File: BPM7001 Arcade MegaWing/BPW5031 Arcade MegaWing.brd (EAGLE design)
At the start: 85.1 x 71.4 mm, 61 parts, among them SW1 TPA-5POS

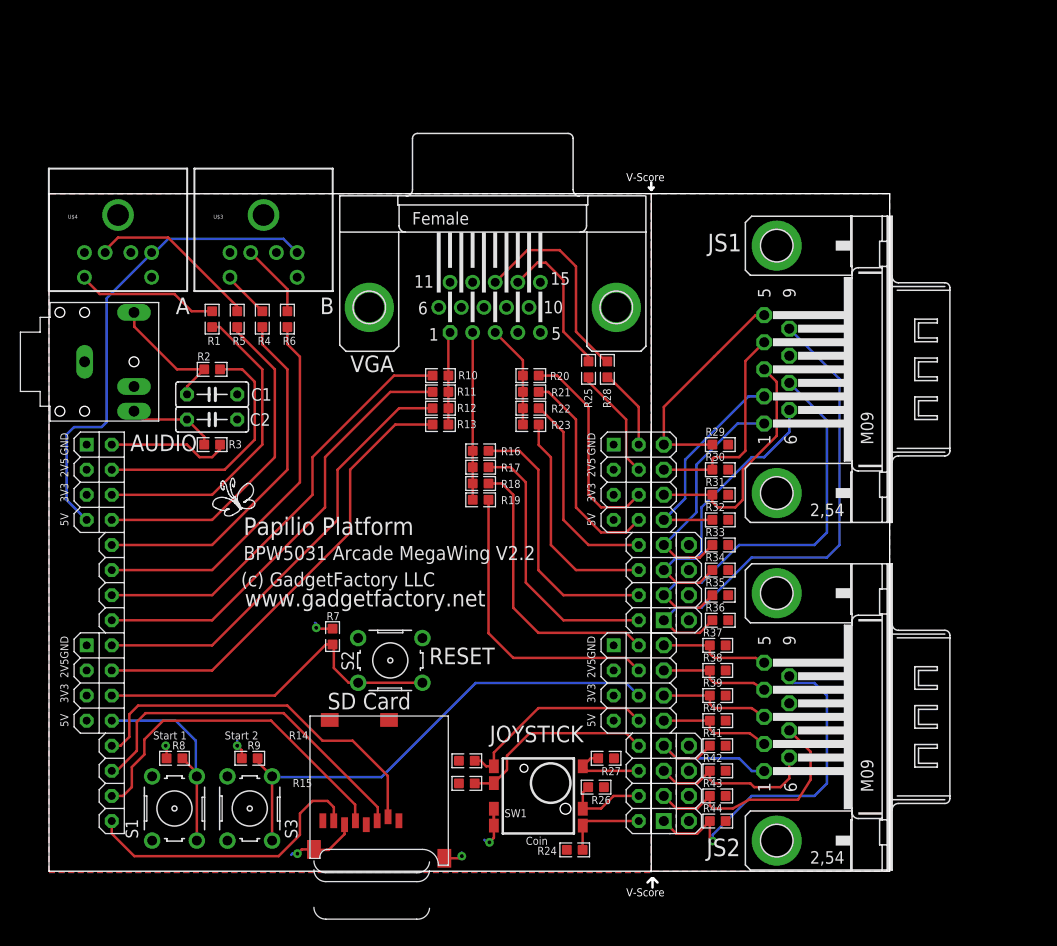
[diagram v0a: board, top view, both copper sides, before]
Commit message: Arcade MegaWing V1.3
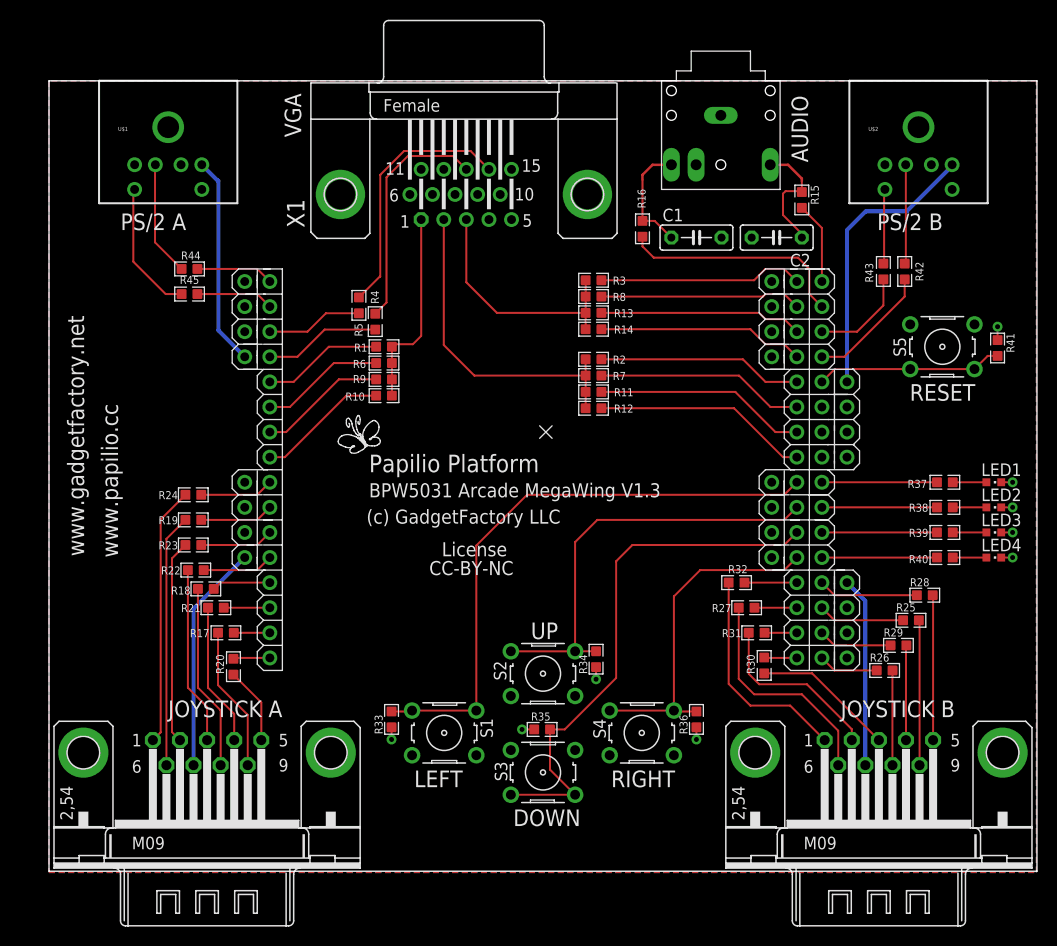
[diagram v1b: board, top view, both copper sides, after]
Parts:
- removed AH, AL: WING8WING8_NOHOLES, Papilio:WINGSIDE_8BIT_NOHOLES
- removed AUDIO1: AUDIOJACK, GadgetFactory:AUDJCK
- removed LOGO1: BUTTERFLY_LOGO, GadgetFactory_Pub:BUTTERFLY_LOGO
- removed SW1: TPA-5POS, GadgetFactory:TPA-5POS
- removed U$3, U$4: MINI-DIN6PTH, SparkFun-Connectors:MINI-DIN6
- added AUDIO: AUDIOJACK, GadgetFactory_6.0:AUDJCK
- added J1: COCOON_48BIT_WINGSIDE, usb1:COCOON_48BIT_WINGSIDE
- added LED1, LED2, LED3, LED4: (no value), led:CHIPLED_0603
- added LOGO2: BUTTERFLY_LOGO, GadgetFactory_Pub:BUTTERFLY_LOGO
- added R45: 390, GadgetFactory:0603
- added S4, S5: (no value), opto:B3F-10XX
- R1: value 390 -> 3.9K
- R10: value 3.9K -> 510
- R11: value 2K -> 1K
- R12: value 1K -> 510
- R13: value 510 -> 1K
- R14: value 47K -> 510
- R15: value 47K -> 3.3K
- R16: value 3.9K -> 3.3K
- R17, R21: value 2K -> 390
- R18, R22: value 1K -> 390
- R19, R23: value 510 -> 390
- R2, R3: value 3.3K -> 3.9K
- R20: value 3.9K -> 390
- R24, R26, R27, R29, R30, R31, R32, R37, R38, R39, R40, R42, R43, R44: value 47K -> 390
- R25, R28: value 82.5 -> 390
- R4, R5: value 390 -> 82.5
- R6: value 390 -> 2K
- R7, R8: value 47K -> 2K
- R9: value 47K -> 1K
- U$1: value MEGAWING_HALF_P1 -> MINI-DIN6PTH; device Papilio:MEGAWING_HALF_NOHOLES_P1 -> SparkFun-Connectors:MINI-DIN6
- U$2: value MICROSD -> MINI-DIN6PTH; device adafruit:MICROSD -> SparkFun-Connectors:MINI-DIN6
- X1: device GadgetFactory:HDF15H -> GadgetFactory_6.0:HDF15H
- moved U$2 89.0 mm to (88.0, 80.0)
- moved U$1 80.9 mm to (12.1, 80.0)
- moved R44 77.3 mm to (14.2, 61.0), turned to 180 degrees
- moved JS1 69.5 mm to (16.0, 12.0), turned to 0 degrees
- moved R15 68.1 mm to (76.2, 67.9), turned to 270 degrees
- moved R8 63.1 mm to (55.1, 58.2), turned to 180 degrees
- moved C2 60.0 mm to (73.7, 64.1), turned to 180 degrees
- moved R43 55.7 mm to (84.5, 60.7), turned to 90 degrees
- moved R42 54.0 mm to (86.6, 60.7), turned to 90 degrees
- moved R24 52.7 mm to (14.6, 38.1), turned to 180 degrees
- moved C1 51.5 mm to (65.5, 64.1)
- moved R41 49.2 mm to (96.0, 53.0), turned to 270 degrees
- moved R14 45.5 mm to (55.1, 54.9), turned to 180 degrees
- moved R20 42.1 mm to (18.7, 20.7), turned to 270 degrees
- moved R3 42.0 mm to (55.1, 59.8), turned to 180 degrees
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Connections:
- removed net BLUE0: R20.1, U$1.A19
- removed net GREEN0: R16.1, U$1.A23
- removed net JOY_3V3: AH.3V3@2, AL.3V3@2, R29.2, R30.2, R31.2, R32.2, R33.2, R34.2, R35.2, R36.2, R37.2, R38.2, R39.2, R40.2, R41.2, R42.2, R43.2, R44.2
- removed net JOY_DOWN: R24.2, SW1.4, U$1.A32
- removed net JOY_FIRE1: R8.2, S1.3, S1.4, U$1.A44
- removed net JOY_FIRE2: R9.2, S3.3, S3.4, U$1.A27
- removed net JOY_GND: AH.GND@2, AL.GND@2, JS1.8, JS2.8
- removed net JOY_LEFT: R14.2, SW1.7, U$1.A28
- removed net JOY_RIGHT: R15.2, SW1.6, U$1.A29
- removed net JOY_SEL: R27.2, SW1.5, U$1.A30
- removed net JOY_UP: R26.2, SW1.3, U$1.A31
- removed net N$2: AH.4, JS1.2, R32.1
- removed net N$24: AH.0, JS1.9, R36.1
- removed net N$7: AH.7, JS1.5, R29.1
- removed net N$8: AH.2, JS1.6, R34.1
- removed net RED0: R10.1, U$1.A39
- removed net SD_!CS: U$1.A45, U$2.2
- removed net SD_DI: U$1.A46, U$2.3
- removed net SD_DO: U$1.A48, U$2.7
- removed net SD_SCK: U$1.A47, U$2.5
- new net BLUE4: J1.B4@1, R14.1
- new net GREEN4: J1.B8@1, R12.1
- new net JS1_1: J1.B13@1, R32.1
- new net JS1_2: J1.B15@1, R31.1
- new net JS1_3: J1.B16@1, R30.1
- new net JS1_4: J1.A2@1, R29.1
- new net JS1_5: J1.A4@1, R28.1
- new net JS1_6: J1.B14@1, R27.1
- new net JS1_8: J1.A1@1, R26.1
- new net JS1_9: J1.A3@1, R25.1
- new net JS2_1: J1.A9@2, R24.1
- new net JS2_2: J1.A11@2, R23.1
- new net JS2_3: J1.A12@2, R22.1
- new net JS2_4: J1.A14@2, R21.1
- new net JS2_5: J1.A16@2, R20.1
- new net JS2_6: J1.A10@2, R19.1
- new net JS2_8: J1.A13@2, R18.1
- new net JS2_9: J1.A15@2, R17.1
- new net LED1: J1.A8@1, R37.2
- new net LED2: J1.A7@1, R38.2
- new net LED3: J1.A6@1, R39.2
- new net LED4: J1.A5@1, R40.2
- new net N$32: JS1.1, R24.2
- new net N$33: JS1.2, R23.2
- new net N$34: JS1.3, R22.2
- new net N$35: JS1.4, R21.2
- new net N$36: JS1.5, R20.2
- new net N$37: JS1.9, R17.2
- new net N$38: JS1.6, R19.2
- new net N$39: JS1.8, R18.2
- new net RED4: J1.A8@2, R10.1
- new net SW1: J1.B9@1, R33.2, S1.3, S1.4
- new net SW2: J1.B10@1, R34.2, S2.3, S2.4
- new net SW3: J1.B11@1, R35.2, S3.3, S3.4
- new net SW4: J1.B12@1, R36.2, S4.3, S4.4
- net 3V3: now also J1.3V3W1@1, J1.3V3W1@2, J1.3V3W1@3, J1.3V3W1@4, J1.3V3W2@1, J1.3V3W2@2, S4.2, S5.2; no longer R14.1, R15.1, R24.1, R26.1, R27.1, U$1.W2_3V3, U$1.W2_3V3_3, U$1.W3_3V3, U$1.W3_3V3_2, U$2.4
- net 5V0: now also J1.VIW1@1, J1.VIW1@2, J1.VIW1@3, J1.VIW1@4, J1.VIW2@1, J1.VIW2@2, JS1.7, JS2.7, U$1.4, U$2.4; no longer U$1.W3_5V, U$3.4, U$4.4
- net AUDIO+: now also J1.A15@1, R16.2; no longer R3.2, U$1.A33
- net AUDIO-: now also J1.A16@1, R15.2; no longer R2.2, U$1.A34
- net BLUE: now also R13.2, R14.2, R3.2, R8.2; no longer R20.2, R21.2, R22.2, R23.2
- net BLUE1: now also J1.B1@1, R3.1; no longer R21.1, U$1.A20
- net BLUE2: now also J1.B2@1, R8.1; no longer R22.1, U$1.A21
- net BLUE3: now also J1.B3@1, R13.1; no longer R23.1, U$1.A22
- net GND: now also AUDIO.1, J1.GNDW1@1, J1.GNDW1@2, J1.GNDW1@3, J1.GNDW1@4, J1.GNDW2@1, J1.GNDW2@2, LED1.C, LED2.C, LED3.C, LED4.C, R33.1, R34.1, R35.1, R36.1, R41.1, U$1.3, U$2.3; no longer AUDIO1.1, R7.1, R8.1, R9.1, SW1.1, SW1.2, U$1.W2_GND, U$1.W2_GND_3, U$1.W3_GND, U$1.W3_GND_2, U$2.6, U$2.MT1, U$2.MT2, U$3.3, U$4.3
- net GREEN: now also R11.2, R12.2, R2.2, R7.2; no longer R16.2, R17.2, R18.2, R19.2
- net GREEN1: now also J1.B5@1, R2.1; no longer R17.1, U$1.A24
- net GREEN2: now also J1.B6@1, R7.1; no longer R18.1, U$1.A25
- net GREEN3: now also J1.B7@1, R11.1; no longer R19.1, U$1.A26
- net HORIZONTAL_SYNC: now also J1.A4@2, R4.1; no longer R28.1, U$1.A17
- net N$1: now also AUDIO.3, C2.1, R15.1; no longer AH.3, JS1.1, R33.1
- net N$10: now also LED3.A, R39.1; no longer AUDIO1.2, C2.1, R3.1
- net N$11: now also LED4.A, R40.1; no longer AUDIO1.3, C1.1, R2.1
- net N$12: now also R42.2, U$2.1; no longer R6.2, U$3.1
- net N$13: now also R43.2, U$2.5; no longer R5.2, U$3.5
- net N$14: now also R44.2, U$1.1; no longer R4.2, U$4.1
- net N$15: now also R45.2, U$1.5; no longer R1.2, U$4.5
- net N$16: now also R32.2; no longer AL.3, R41.1
- net N$17: now also R31.2; no longer AL.4, R40.1
- net N$18: now also R30.2; no longer AL.5, R39.1
- net N$19: now also R29.2; no longer AL.6, R38.1
- net N$20: now also R28.2; no longer AL.7, R37.1
- net N$21: now also JS2.9, R25.2; no longer AL.2, JS2.6, R42.1
- net N$22: now also JS2.6, R27.2; no longer AL.1, JS2.7, R43.1
- net N$23: now also JS2.8, R26.2; no longer AL.0, JS2.9, R44.1
- net N$3: now also LED1.A, R37.1; no longer AH.5, JS1.3, R31.1
- net N$4: now also R4.2; no longer R28.2
- net N$5: now also R5.2; no longer R25.2
- net N$6: now also AUDIO.2, C1.1, R16.1; no longer AH.6, JS1.4, R30.1
- net N$9: now also LED2.A, R38.1; no longer AH.1, JS1.7, R35.1
- net PS2CLK1: now also J1.A14@1, R43.1; no longer R5.1, U$1.A37
- net PS2CLK2: now also J1.A2@2, R45.1; no longer R1.1, U$1.A35
- net PS2DAT1: now also J1.A13@1, R42.1; no longer R6.1, U$1.A38
- net PS2DAT2: now also J1.A1@2, R44.1; no longer R4.1, U$1.A36
- net RED: now also R1.2, R6.2, R9.2; no longer R11.2, R12.2, R13.2
- net RED1: now also J1.A5@2, R1.1; no longer R11.1, U$1.A40
- net RED2: now also J1.A6@2, R6.1; no longer R12.1, U$1.A41
- net RED3: now also J1.A7@2, R9.1; no longer R13.1, U$1.A42
- net RESET: now also J1.A12@1, R41.2, S5.3, S5.4; no longer R7.2, S2.3, S2.4, U$1.A43
- net VERTICAL_SYNC: now also J1.A3@2, R5.1; no longer R25.1, U$1.A18
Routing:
- net SW1: track 0.00 -> 60.4 mm
- net SW3: track 0.00 -> 54.3 mm
- net N$24: track 50.9 -> 0.00 mm
- net JOY_FIRE2: track 50.5 -> 0.00 mm
- net RED0: track 43.9 -> 0.00 mm
- net SW2: track 0.00 -> 43.6 mm
- net 5V0: track 49.0 -> 92.5 mm
- net N$9: track 41.8 -> 3.40 mm
- net SD_!CS: track 38.1 -> 0.00 mm
- net SD_DI: track 36.4 -> 0.00 mm
- net SD_SCK: track 35.0 -> 0.00 mm
- net SW4: track 0.00 -> 35.0 mm
- net RED3: track 46.5 -> 13.0 mm
- net RED1: track 45.0 -> 12.2 mm
- net RED2: track 45.4 -> 12.6 mm
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- removed copper zone on layer 1, net JOY_3V3
- removed copper zone on layer 16, net JOY_GND
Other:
- board size 85.1 x 71.4 mm -> 100 x 80 mm
- board text added: "BPW5031 Arcade MegaWing V1.3"
- board text added: "CC-BY-NC"
- board text added: "DOWN"
- board text added: "JOYSTICK A"
- board text added: "JOYSTICK B"
- board text added: "LEFT"
- board text added: "License"
- board text added: "PS/2 A"
- board text added: "PS/2 B"
- board text added: "RIGHT"
- board text added: "UP"
- board text added: "www.papilio.cc"
- board text removed: "A"
- board text removed: "B"
- board text removed: "BPW5031 Arcade MegaWing V2.2"
- board text removed: "Coin"
- board text removed: "JOYSTICK"
- board text removed: "SD Card"
- board text removed: "Start 1"
- board text removed: "Start 2"
- board text removed: "V-Score"
